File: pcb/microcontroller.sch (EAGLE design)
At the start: 8 parts

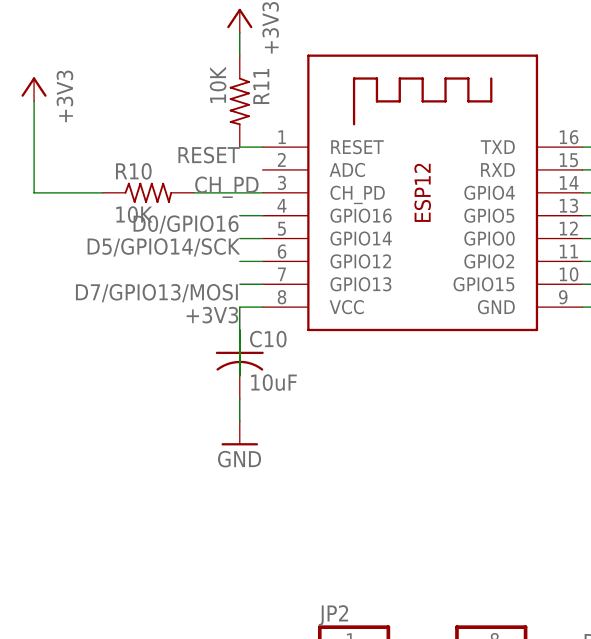
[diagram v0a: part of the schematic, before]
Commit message: microcontroller board ready to be fab'd
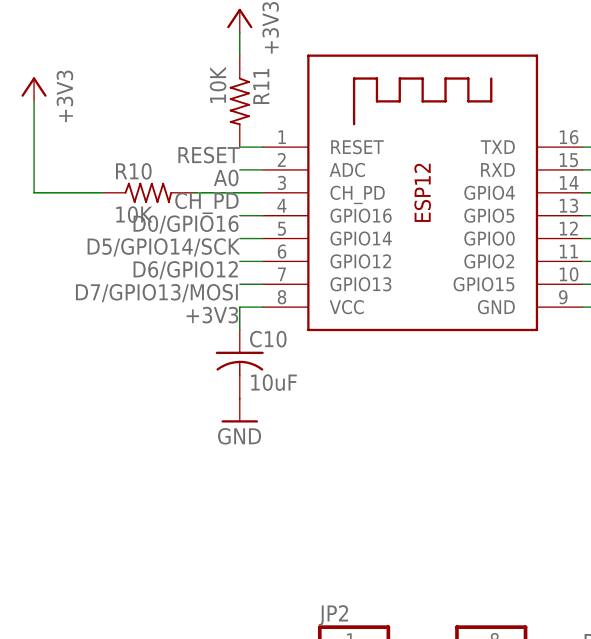
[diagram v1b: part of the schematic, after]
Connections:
- removed net N$2: X1.GPIO12
- net A0: now also X1.ADC
- net D6/GPIO12: now also X1.GPIO12
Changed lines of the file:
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@@
 <attribute name="VALUE" x="122.936" y="44.069" size="1.778" layer="96"/>
 </instance>
-<instance part="GND11" gate="1" x="121.92" y="38.1" smashed="yes">
-<attribute name="VALUE" x="119.38" y="35.56" size="1.778" layer="96"/>
+<instance part="GND11" gate="1" x="121.92" y="40.64" smashed="yes">
+<attribute name="VALUE" x="119.38" y="38.1" size="1.778" layer="96"/>
 </instance>
 <instance part="+3V4" gate="G$1" x="180.34" y="76.2" smashed="yes" rot="MR0">
@@
 <pinref part="C10" gate="G$1" pin="2"/>
 <pinref part="GND11" gate="1" pin="GND"/>
-<wire x1="121.92" y1="43.18" x2="121.92" y2="40.64" width="0.1524" layer="91"/>
 </segment>
 <segment>
@@
 <pinref part="X1" gate="G$1" pin="VCC"/>
 <pinref part="C10" gate="G$1" pin="1"/>
-<wire x1="121.92" y1="45.72" x2="121.92" y2="50.8" width="0.1524" layer="91"/>
-<wire x1="121.92" y1="45.72" x2="121.92" y2="53.34" width="0.1524" layer="91"/>
+<wire x1="121.92" y1="50.8" x2="121.92" y2="53.34" width="0.1524" layer="91"/>
 </segment>
 <segment>
@@
 <wire x1="124.46" y1="66.04" x2="116.84" y2="66.04" width="0.1524" layer="91"/>
 <pinref part="X1" gate="G$1" pin="CH_PD"/>
-<label x="116.84" y="66.04" size="1.778" layer="95"/>
+<label x="121.92" y="66.04" size="1.778" layer="95" rot="R180"/>
 </segment>
 </net>
@@
 <label x="160.02" y="5.08" size="1.778" layer="95"/>
 </segment>
+<segment>
+<pinref part="X1" gate="G$1" pin="GPIO12"/>
+<wire x1="124.46" y1="58.42" x2="121.92" y2="58.42" width="0.1524" layer="91"/>
+<label x="121.92" y="58.42" size="1.778" layer="95" rot="R180"/>
+</segment>
 </net>
 <net name="D5/GPIO14/SCK" class="0">
@@
 <label x="160.02" y="12.7" size="1.778" layer="95"/>
 </segment>
+<segment>
+<pinref part="X1" gate="G$1" pin="ADC"/>
+<wire x1="124.46" y1="68.58" x2="121.92" y2="68.58" width="0.1524" layer="91"/>
+<label x="121.92" y="68.58" size="1.778" layer="95" rot="R180"/>
+</segment>
 </net>
 <net name="D7/GPIO13/MOSI" class="0">
@@
 </segment>
 </net>
-<net name="N$2" class="0">
-<segment>
-<pinref part="X1" gate="G$1" pin="GPIO12"/>
-<wire x1="124.46" y1="58.42" x2="121.92" y2="58.42" width="0.1524" layer="91"/>
-</segment>
-</net>
 </nets>
 </sheet>
 </sheets>
-<errors>
-</errors>
 </schematic>
 </drawing>
